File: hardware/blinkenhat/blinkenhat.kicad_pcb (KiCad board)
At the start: 2 copper layers, 58.9 x 27.9 mm, 26 parts, among them J1 LED1, J2 LED2, J3 INPUT, J4 Programmer, J5 USB_POWER, J6 GPIO, Q1 2N7002, Q2 2N7002, SW1 RESET, U1 AMS1117-3V3, U2 ESP-12E

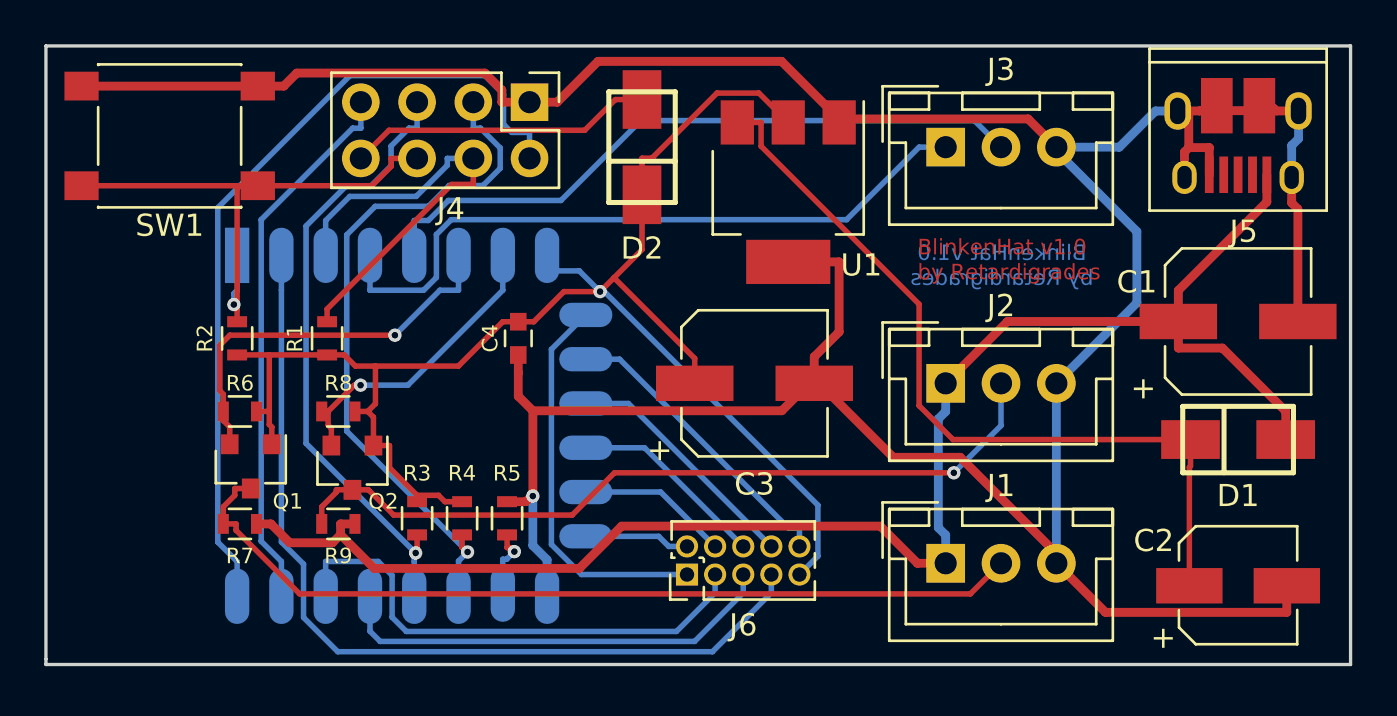
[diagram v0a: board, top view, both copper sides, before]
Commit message: Hardware: redesign PCB.
Signed-off-by: Jan Losinski <losinski@wh2.tu-dresden.de>
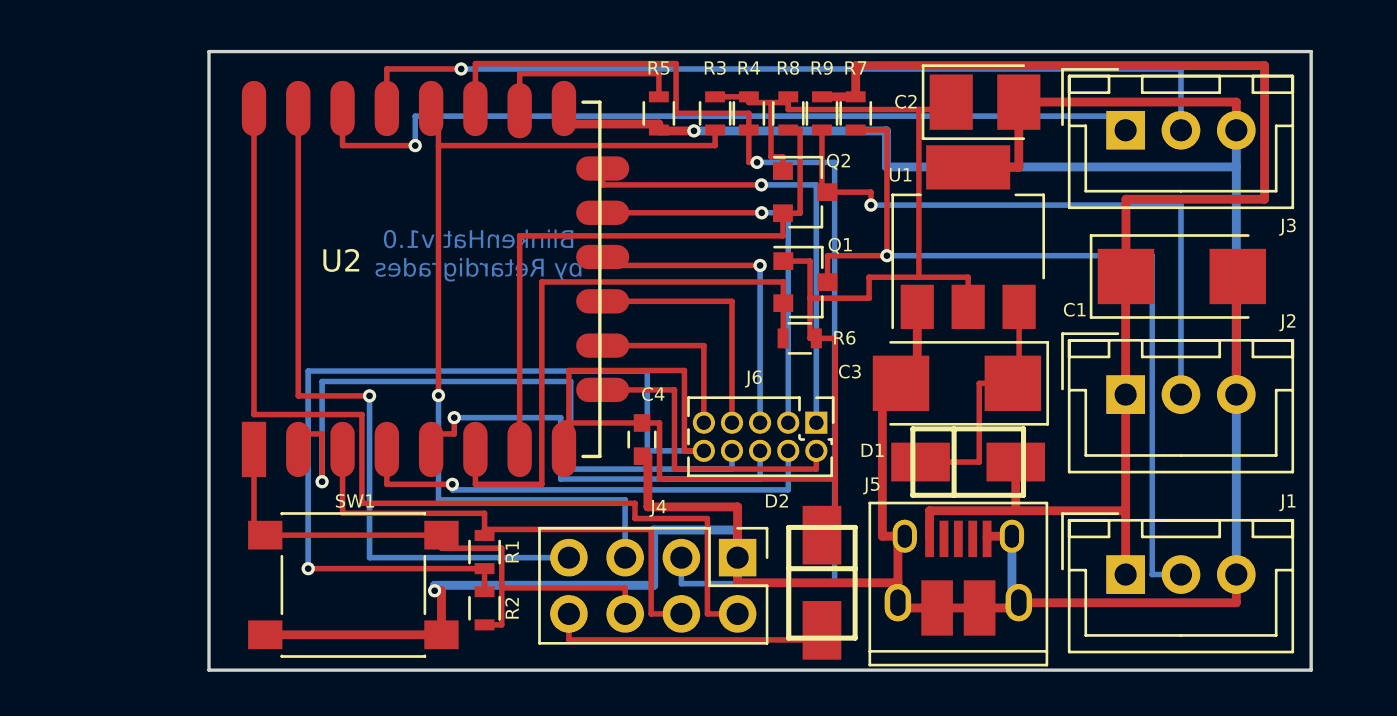
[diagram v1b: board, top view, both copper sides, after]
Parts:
- C1: value 100µ -> 200µ; footprint Capacitors_SMD:CP_Elec_6.3x5.8 -> Capacitors_Tantalum_SMD:CP_Tantalum_Case-C_EIA-6032-28_Reflow
- C2: footprint Capacitors_SMD:CP_Elec_5x5.3 -> Capacitors_Tantalum_SMD:CP_Tantalum_Case-B_EIA-3528-21_Reflow
- C3: footprint Capacitors_SMD:CP_Elec_6.3x5.8 -> Capacitors_Tantalum_SMD:CP_Tantalum_Case-C_EIA-6032-28_Reflow
- U2: moved to F.Cu
- moved R7 33.4 mm to (145.5, 88.6), turned to 270 degrees
- moved R9 28.7 mm to (144.0, 88.6), turned to 270 degrees
- moved Q1 26.4 mm to (143.3, 96.3), turned to 0 degrees
- moved R6 25.5 mm to (143.0, 98.8)
- moved C2 24.7 mm to (151.4, 88.1)
- moved R8 24.4 mm to (142.5, 88.6), turned to 270 degrees
- moved Q2 23.9 mm to (143.3, 92.2), turned to 0 degrees
- moved J5 23.2 mm to (150.2, 109.4), turned to 0 degrees
- moved R3 22.7 mm to (139.2, 88.6)
- moved J4 22.6 mm to (140.2, 108.7)
- moved R4 22.4 mm to (140.7, 88.6)
- moved SW1 21.9 mm to (122.9, 109.9), turned to 0 degrees
- moved D2 21.3 mm to (144.0, 109.8), turned to 270 degrees
- moved R5 19.5 mm to (136.7, 88.6), turned to 270 degrees
- moved R2 16.5 mm to (128.8, 111.0), turned to 270 degrees
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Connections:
- C2 pad 1: Net-(C2-Pad1) -> +3V3
- C3 pad 1: +3V3 -> Net-(C3-Pad1)
- D1 pad 1: Net-(C2-Pad1) -> Net-(C3-Pad1)
- J3 pad 1: INP1 -> INP2
- J3 pad 2: INP2 -> INP1
- J6 pad 1: CSO -> SCLK
- J6 pad 10: MISO -> +3V3
- J6 pad 2: SCLK -> CSO
- J6 pad 3: GPIO5 -> MOSI
- J6 pad 4: MOSI -> GPIO16
- J6 pad 5: GPIO4 -> GPIO10
- J6 pad 6: GPIO10 -> GPIO15
- J6 pad 7: ADC -> GPIO9
- J6 pad 8: GPIO9 -> ADC
- J6 pad 9: +3V3 -> MISO
- U1 pad 3: Net-(C2-Pad1) -> Net-(C3-Pad1)
- U2 pad 13: GPIO4 -> INP1
- U2 pad 14: GPIO5 -> INP2
- U2 pad 4: INP1 -> GPIO16
- U2 pad 5: INP2 -> GPIO15
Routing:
- net +3V3: track 74.6 -> 114.6 mm
- net Net-(C2-Pad1): track 36.3 -> 0.00 mm
- net GPIO5: track 22.4 -> 0.00 mm
- net GPIO16: track 0.00 -> 22.4 mm, vias 0 -> 1
- net GPIO4: track 21.1 -> 0.00 mm
- net GPIO2: track 30.8 -> 50.5 mm
- net GPIO15: track 0.00 -> 19.6 mm, vias 0 -> 1
- net SCLK: track 4.76 -> 21.1 mm, vias 0 -> 1
- net GPIO0: track 27.5 -> 41.6 mm
- net LED2: track 12.9 -> 26.9 mm, vias 1 -> 0
- net Net-(C3-Pad1): track 0.00 -> 11.5 mm
- net MOSI: track 6.86 -> 17.9 mm, vias 0 -> 1
- net LED1: track 17.3 -> 27.9 mm, vias 1 -> 0
- net INP1: track 30.7 -> 41.1 mm, vias 0 -> 1
- net +5V: track 71.7 -> 63.0 mm
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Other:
- board size 58.9 x 27.9 mm -> 49.8 x 27.9 mm
